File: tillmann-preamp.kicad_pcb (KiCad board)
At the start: 2 copper layers, 35 x 40.6 mm, 12 parts, among them J1 AudioJack3_Switch, J2 Input Signal, J4 AudioJack3_Switch, J4 Output Signal, J5 Barrel_Jack, Q1 Q_NJFET_DGS

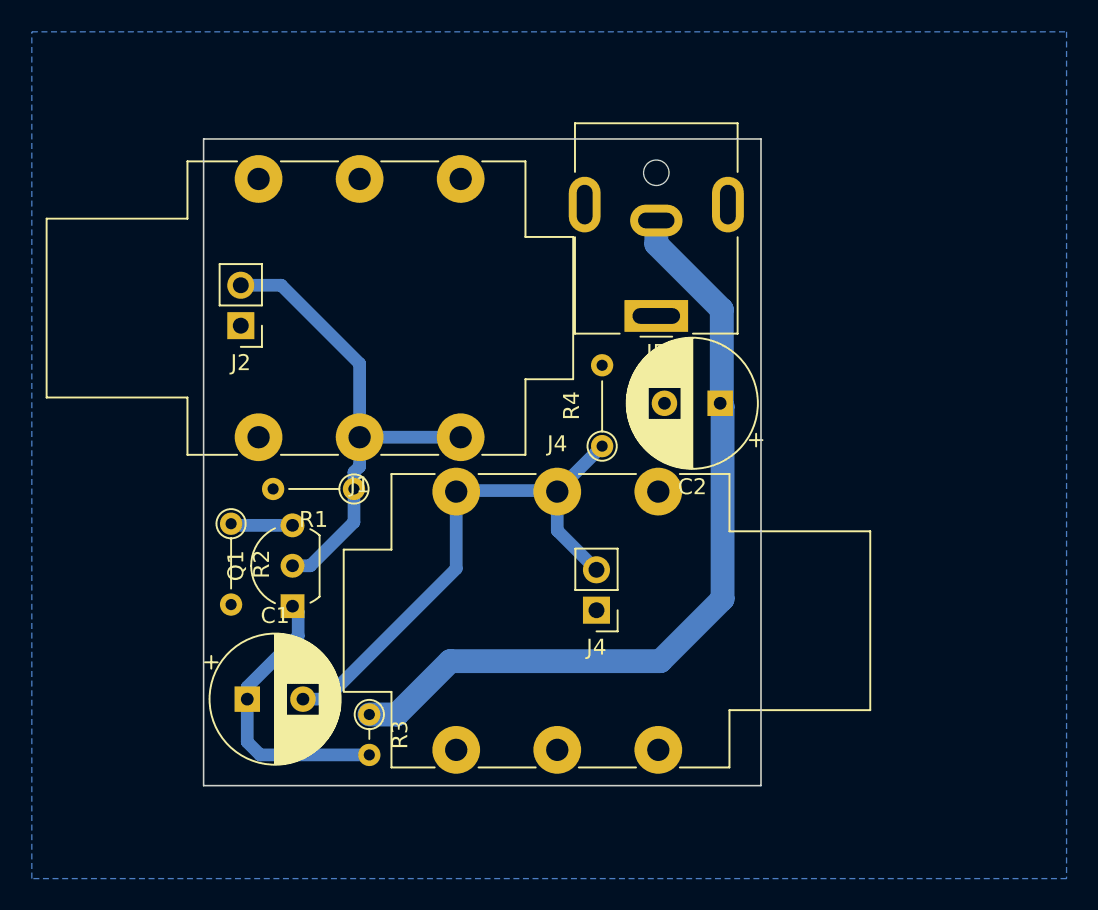
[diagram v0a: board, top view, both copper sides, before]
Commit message: Update PCB for milling v1.0
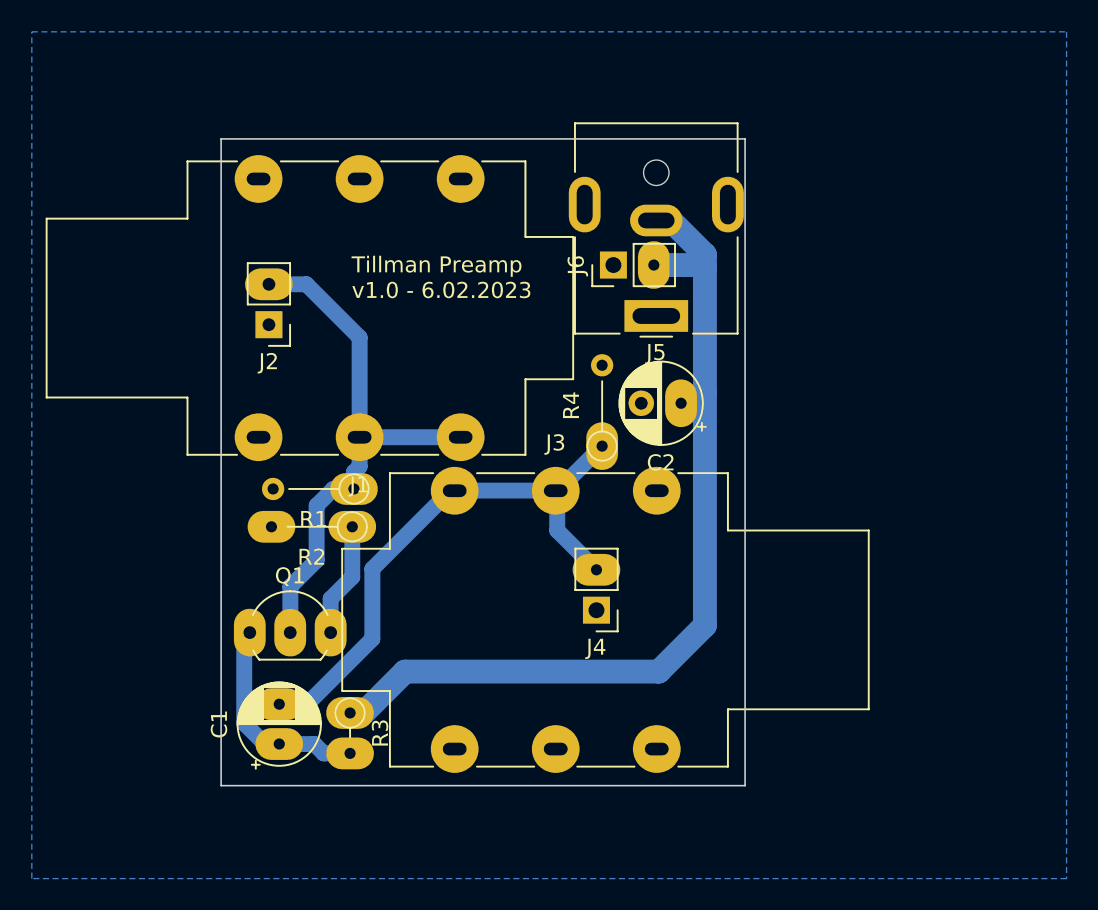
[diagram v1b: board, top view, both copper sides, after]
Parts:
- removed the J4 at (110.9, 103.2)
- added J3: AudioJack3_Switch, Connector_Audio:Jack_6.35mm_Neutrik_NMJ6HFD2-AU_Horizontal, F.Cu at (110.8, 103.1)
- added J6: 9V, Connector_PinHeader_2.54mm:PinHeader_1x02_P2.54mm_Vertical, F.Cu at (120.8, 89.0)
- C1, C2: footprint Capacitor_THT:CP_Radial_D8.0mm_P3.50mm -> Capacitor_THT:CP_Radial_D5.0mm_P2.50mm
- moved R2 7.62 mm to (104.3, 105.4), turned to 180 degrees
- moved C1 3.46 mm to (99.8, 119.0), turned to 90 degrees
- moved Q1 3.16 mm to (97.9, 112.0), turned to 0 degrees
- moved C2 2.46 mm to (125.0, 97.6)
- moved J2 1.77 mm to (99.1, 92.7)
- moved R3 1.21 mm to (104.2, 117.1)
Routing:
- net Net-(C1-Pad2): track 34.3 -> 41.9 mm
- net +9V: track 50.9 -> 56.9 mm
- net Net-(C1-Pad1): track 18.0 -> 13.3 mm
- net Net-(J1-PadR): track 31.0 -> 34.6 mm
- net Net-(Q1-Pad3): track 3.90 -> 7.21 mm
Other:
- board size 35 x 40.6 mm -> 32.9 x 40.6 mm
- board text added: "Tillman Preamp v1.0 - 6.02.2023"
